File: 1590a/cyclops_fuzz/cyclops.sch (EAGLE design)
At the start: 44 parts, among them IC1 4558, IC2 741

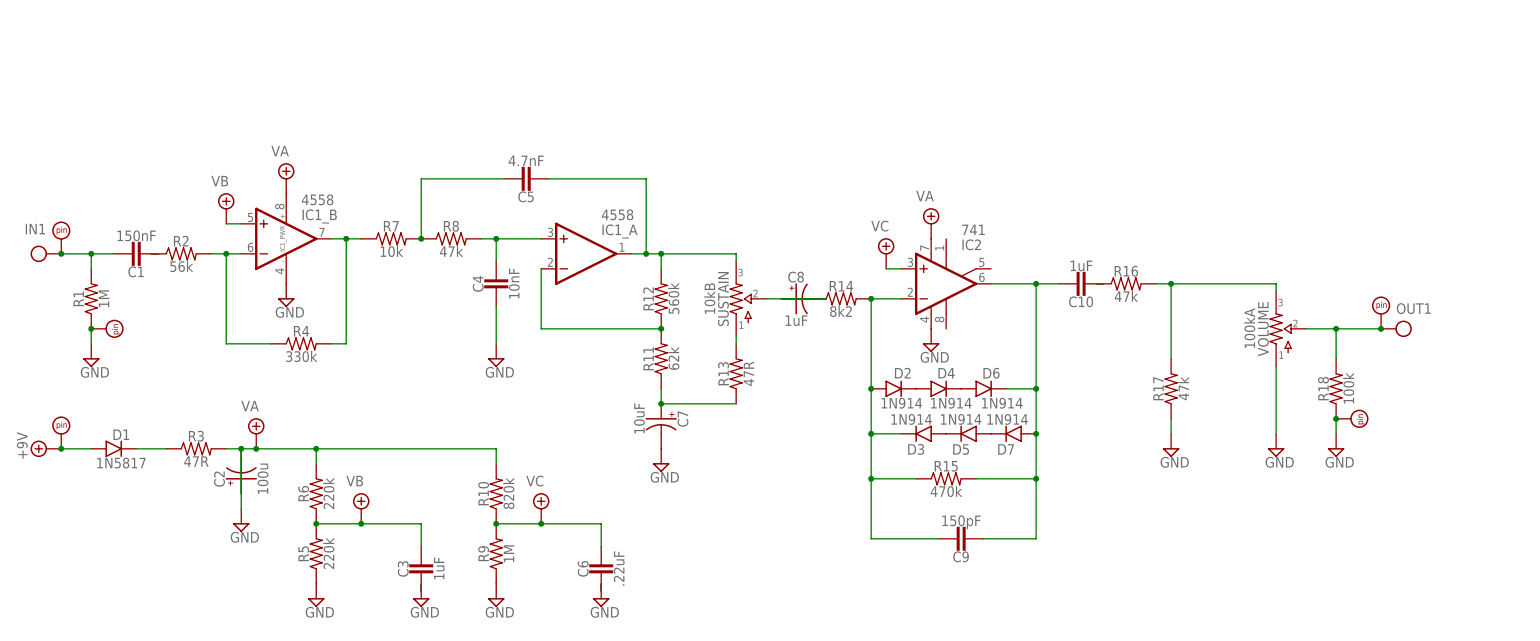
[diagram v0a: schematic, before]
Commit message: updates to cerberus and cyclops
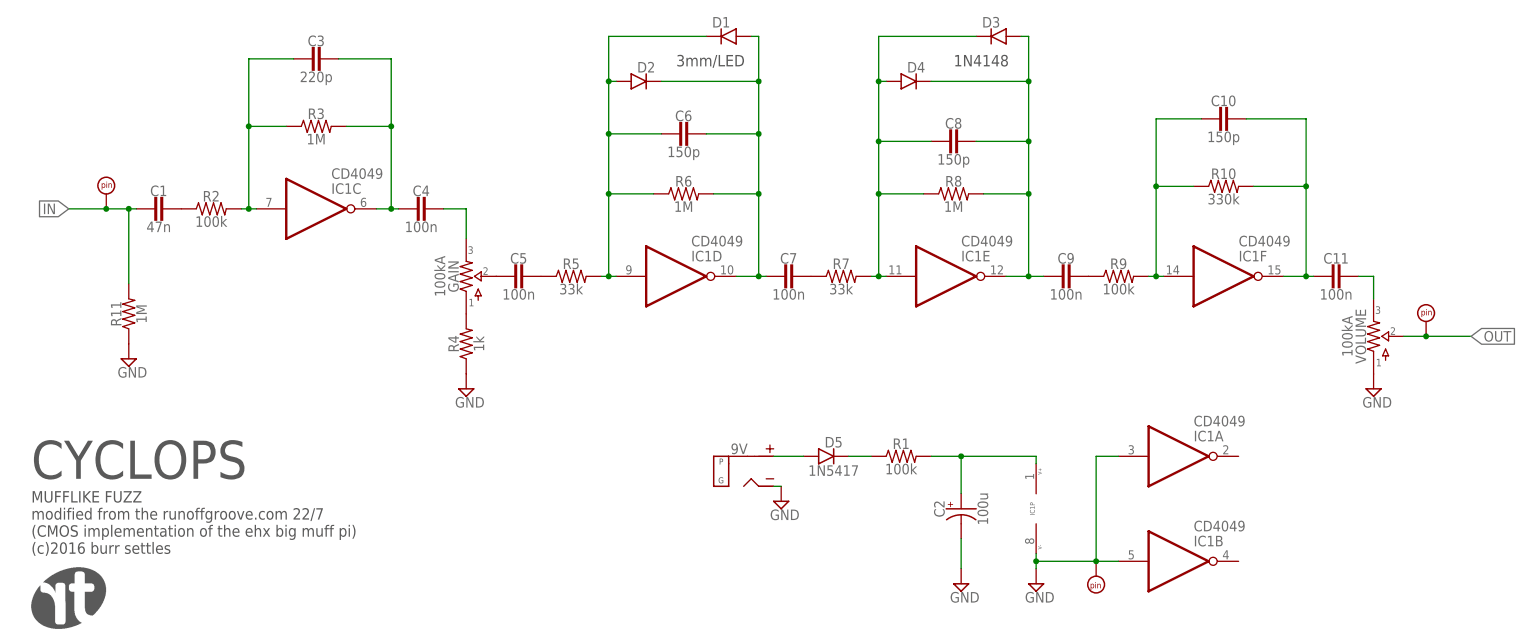
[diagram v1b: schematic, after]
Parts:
- removed D6, D7: 1N914, diodes:DO35.2
- removed IC2: 741, integrated circuits:SINGLETH
- removed PAD1, PAD2, PAD5: PADSQR, supply pins:PADSQR
- removed PAD3, PAD4: PADRND, supply pins:PADRND
- removed R12: 560k, resistors:R_.2
- removed R13: 47R, resistors:R_.2
- removed R14: 8k2, resistors:R_.2
- removed R15: 470k, resistors:R_.2
- removed R16, R17: 47k, resistors:R_.2
- removed R18: 100k, resistors:R_.2
- removed SUSTAIN: 10kB, potentiometers:POTSTRIM
- added 9V: DC_MONO, jacks:DC_MONO
- added C11: 100n, capacitors-film:CER/FILM2
- added GAIN: 100kA, potentiometers:POTSTRIM
- added GND: PADRND, supply pins:PADRND
- added IN, OUT: PADSQR, supply pins:PADSQR
- C1: value 150nF -> 47n; device capacitors-film:CER/FILMBOX.1 -> capacitors-film:CER/FILM2
- C10: value 1uF -> 150p; device capacitors-film:CER/FILMBOX.2 -> capacitors-film:CER/FILM2
- C3: value 1uF -> 220p; device capacitors-film:CER/FILMBOX.2 -> capacitors-film:CER/FILM2
- C4: value 10nF -> 100n; device capacitors-film:CER/FILMBOX.1 -> capacitors-film:CER/FILM2
- C5: value 4.7nF -> 100n; device capacitors-film:CER/FILMBOX.1 -> capacitors-film:CER/FILM2
- C6: value .22uF -> 150p; device capacitors-film:CER/FILMBOX.1 -> capacitors-film:CER/FILM2
- C7: value 10uF -> 100n; device capacitors-elec:0501 -> capacitors-film:CER/FILM2
- C8: value 1uF -> 150p; device capacitors-elec:0501 -> capacitors-film:CER/FILM2
- C9: value 150pF -> 100n; device capacitors-film:CER/FILMBOX.1 -> capacitors-film:CER/FILM2
- D1: value 1N5817 -> (none)
- D2, D3, D4: value 1N914 -> (none); device diodes:DO35.2 -> diodes:DO41.2
- D5: value 1N914 -> 1N5417; device diodes:DO35.2 -> diodes:DO41.3
- IC1: value 4558 -> CD4049; device integrated circuits:DUALTH -> integrated circuits:CD4049UBE
- R1, R9: value 1M -> 100k
- R10: value 820k -> 330k
- R11: value 62k -> 1M
- R2: value 56k -> 100k
- R3: value 47R -> 1M
- R4: value 330k -> 1k
- R5: value 220k -> 33k
- R6: value 220k -> 1M
- R7: value 10k -> 33k
- R8: value 47k -> 1M
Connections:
- removed net +9V: D1.A, PAD1.P$1
- removed net N$19: D5.A, D7.C
- removed net N$20: D3.A, D5.C
- removed net VA: C2.+, IC1_PWR.V+, IC2.V+, R10.2, R3.2, R6.2
- removed net VB: C3.1, IC1_B.+IN, R5.2, R6.1
- removed net VC: C6.1, IC2.+IN, R10.1, R9.2
- new net N$15: GAIN.1, R4.2
- net GND: now also 9V.SLEEVE, GND.P$1, IC1A.I, IC1B.I, IC1P.VSS, R11.1, R4.1; no longer C3.2, C4.2, C6.2, C7.-, IC1_PWR.V-, IC2.V-, PAD3.P$1, PAD4.P$1, R1.1, R17.1, R18.1, R5.1, R9.1
- net IN: now also C1.2, IN.P$1, R11.2; no longer C1.1, PAD2.P$1, R1.2
- net N$1: now also C3.1, C4.2, IC1C.O, R3.2; no longer C1.2, R2.1
- net N$10: now also C4.1, GAIN.3; no longer C7.+, R11.1, R13.1
- net N$11: now also C8.1, C9.2, D3.A, D4.C, IC1E.O, R8.2; no longer R13.2, SUSTAIN.1
- net N$12: now also C9.1, R9.1; no longer D1.C, R3.1
- net N$13: now also C10.2, IC1F.I, R10.1, R9.2; no longer C8.-, SUSTAIN.2
- net N$14: now also C10.1, C11.2, IC1F.O, R10.2; no longer C8.+, R14.1
- net N$16: now also C11.1, VOLUME.3; no longer C9.1, D2.A, D3.C, IC2.-IN, R14.2, R15.1
- net N$17: now also 9V.TIP, D5.A; no longer D2.C, D4.A
- net N$18: now also C2.+, IC1P.VDD, R1.2; no longer D4.C, D6.A
- net N$2: now also C5.2, GAIN.2; no longer C10.2, R16.1
- net N$21: now also D5.C, R1.1; no longer C10.1, C9.2, D6.C, D7.A, IC2.OUT, R15.2
- net N$3: now also C3.2, IC1C.I, R2.2, R3.1; no longer R16.2, R17.2, VOLUME.3
- net N$4: now also C1.1, R2.1; no longer IC1_B.-IN, R2.2, R4.1
- net N$5: now also C5.1, R5.1; no longer IC1_B.OUT, R4.2, R7.1
- net N$6: now also C6.2, D1.C, D2.A, IC1D.I, R5.2, R6.1; no longer C5.1, R7.2, R8.1
- net N$7: now also C6.1, C7.2, D1.A, D2.C, IC1D.O, R6.2; no longer C4.1, IC1_A.+IN, R8.2
- net N$8: now also C7.1, R7.1; no longer C5.2, IC1_A.OUT, R12.2, SUSTAIN.3
- net N$9: now also C8.2, D3.C, D4.A, IC1E.I, R7.2, R8.1; no longer IC1_A.-IN, R11.2, R12.1
- net OUT: now also OUT.P$1; no longer PAD5.P$1, R18.2
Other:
- note added: "1N4148"
- note added: "3mm/LED"
- note added: "CYCLOPS"
- note added: "MUFFLIKE FUZZ modified from the runoffgroove.com 22/7 (CMOS implementation of the ehx big muff pi) (c)2016 burr settles"
- moved on the sheet: C1, C10, C2, C3, C4, C5, C6, C9, D1, D2, D3, D4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
